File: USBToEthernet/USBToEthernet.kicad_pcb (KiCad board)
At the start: 2 copper layers, 52.4 x 25.3 mm, 54 parts, among them J1 0480372200, J2 L836-1J1T-43, SW1 SW_Push, U1 LAN7500-ABJZ, U2 NCP1117-3.3_SOT223, U3 93LCxxAxxOT, U4 USBLC6-2SC6, U6 AMS1117-1.2, Y1 25Mhz

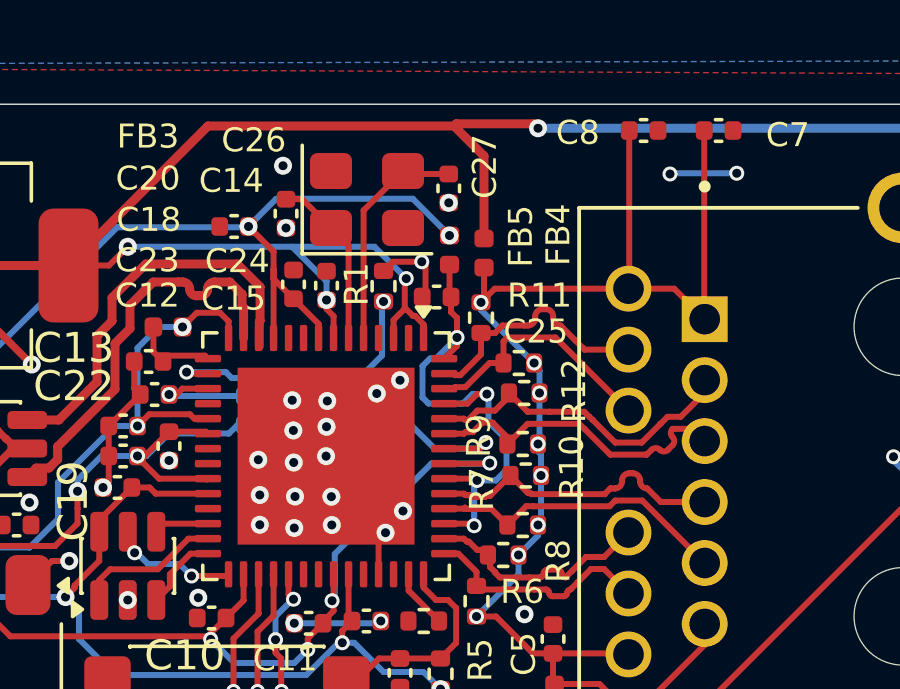
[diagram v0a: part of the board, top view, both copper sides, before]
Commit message: update repo fr
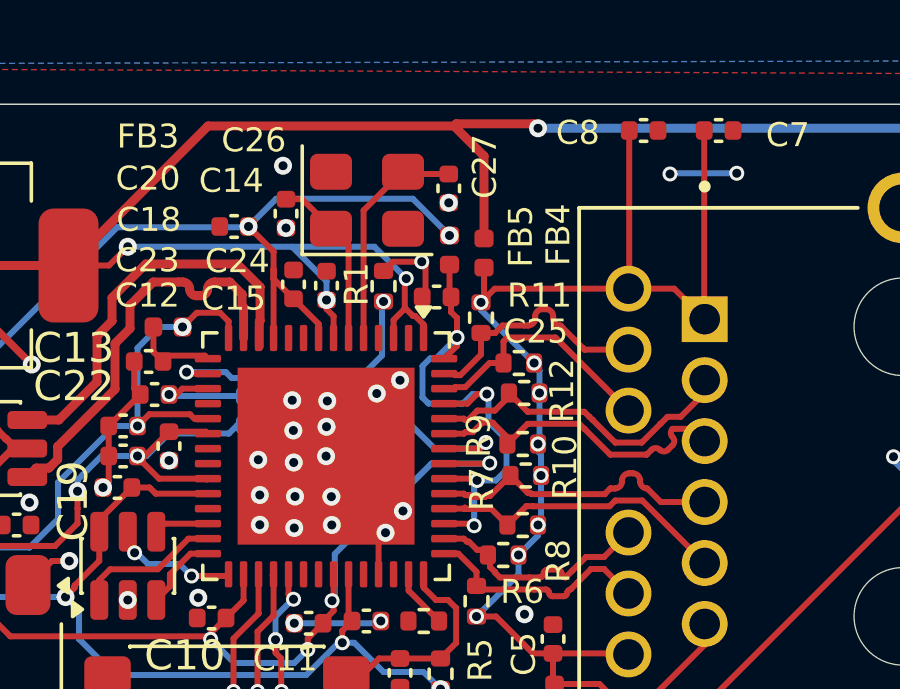
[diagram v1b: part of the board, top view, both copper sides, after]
